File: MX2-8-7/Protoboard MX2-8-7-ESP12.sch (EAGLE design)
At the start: 145 parts, among them X1 ESP-12E

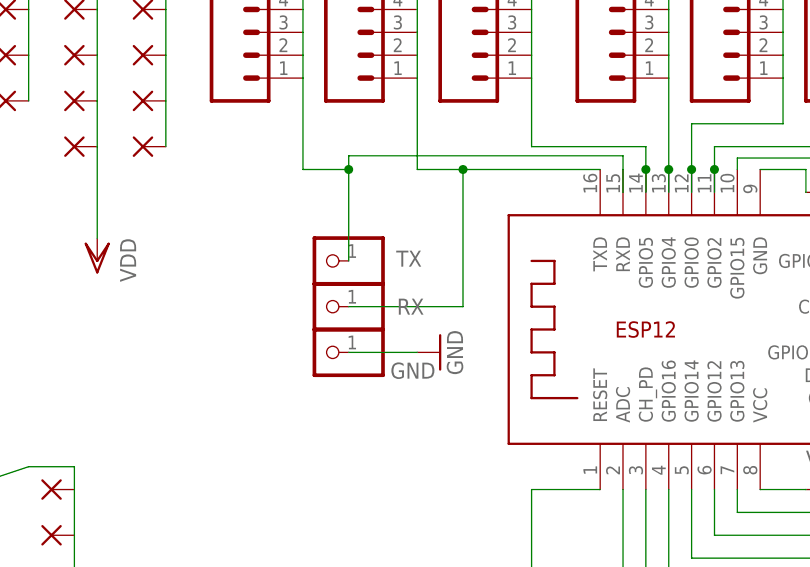
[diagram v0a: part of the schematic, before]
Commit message: Silkscreen text fixes
Silkscreen text fixes
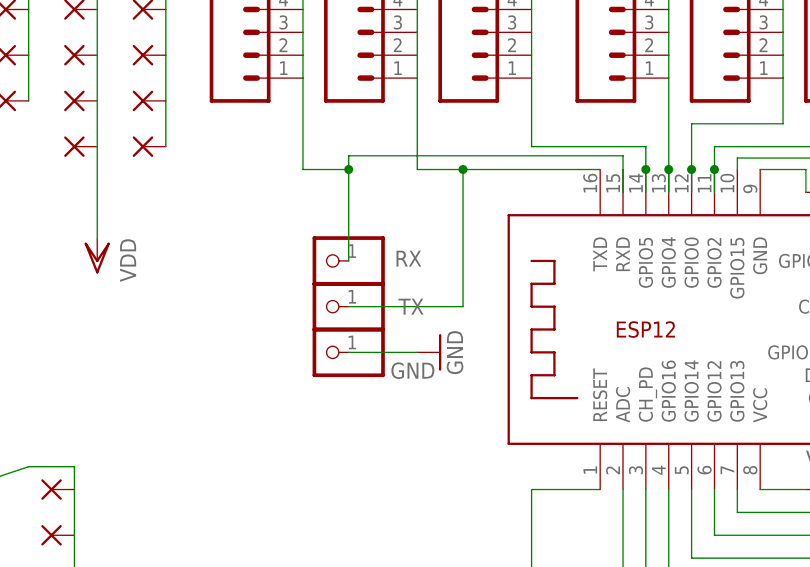
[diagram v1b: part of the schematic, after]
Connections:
- net N$45: now also RX.1; no longer TX.1
- net N$46: now also TX.1; no longer RX.1
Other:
- moved on the sheet: RX, TX
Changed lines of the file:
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@@
 <?xml version="1.0" encoding="utf-8"?>
 <!DOCTYPE eagle SYSTEM "eagle.dtd">
-<eagle version="7.6.0">
+<eagle version="7.7.0">
 <drawing>
 <settings>
@@
 <part name="J29" library="SparkFun-Connectors" deviceset="M05" device="NO_SILK"/>
 <part name="J30" library="SparkFun-Connectors" deviceset="M05" device="NO_SILK"/>
+<part name="RX" library="adafruit" deviceset="PINHD-1X1" device="CB"/>
 <part name="TX" library="adafruit" deviceset="PINHD-1X1" device="CB"/>
-<part name="RX" library="adafruit" deviceset="PINHD-1X1" device="CB"/>
 <part name="GND" library="adafruit" deviceset="PINHD-1X1" device="CB"/>
 <part name="GND6" library="supply1" deviceset="GND" device=""/>
@@
 <instance part="J29" gate="G$1" x="172.72" y="-35.56"/>
 <instance part="J30" gate="G$1" x="330.2" y="-30.48"/>
-<instance part="TX" gate="G$1" x="53.34" y="15.24" smashed="yes" rot="R180">
+<instance part="RX" gate="G$1" x="53.34" y="15.24" smashed="yes" rot="R180">
 <attribute name="NAME" x="64.008" y="16.383" size="1.778" layer="95" rot="R180"/>
 <attribute name="VALUE" x="59.69" y="20.32" size="1.778" layer="96" rot="R180"/>
 </instance>
-<instance part="RX" gate="G$1" x="53.34" y="10.16" smashed="yes" rot="R180">
+<instance part="TX" gate="G$1" x="53.34" y="10.16" smashed="yes" rot="R180">
 <attribute name="NAME" x="64.262" y="11.049" size="1.778" layer="95" rot="R180"/>
 <attribute name="VALUE" x="59.69" y="15.24" size="1.778" layer="96" rot="R180"/>
@@
 <wire x1="83.82" y1="25.4" x2="68.58" y2="25.4" width="0.1524" layer="91"/>
 <wire x1="68.58" y1="25.4" x2="68.58" y2="10.16" width="0.1524" layer="91"/>
-<pinref part="RX" gate="G$1" pin="1"/>
+<pinref part="TX" gate="G$1" pin="1"/>
 <wire x1="68.58" y1="10.16" x2="55.88" y2="10.16" width="0.1524" layer="91"/>
 <pinref part="X1" gate="G$1" pin="TXD"/>
@@
 <wire x1="86.36" y1="22.86" x2="86.36" y2="25.4" width="0.1524" layer="91"/>
 <wire x1="86.36" y1="25.4" x2="86.36" y2="26.924" width="0.1524" layer="91"/>
-<pinref part="TX" gate="G$1" pin="1"/>
+<pinref part="RX" gate="G$1" pin="1"/>
 <wire x1="55.88" y1="26.924" x2="55.88" y2="25.4" width="0.1524" layer="91"/>
 <wire x1="55.88" y1="25.4" x2="55.88" y2="15.24" width="0.1524" layer="91"/>
